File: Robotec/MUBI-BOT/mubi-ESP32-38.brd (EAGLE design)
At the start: 76.5 x 49.5 mm, 20 parts, among them IC1 L293D, IC2 7805T

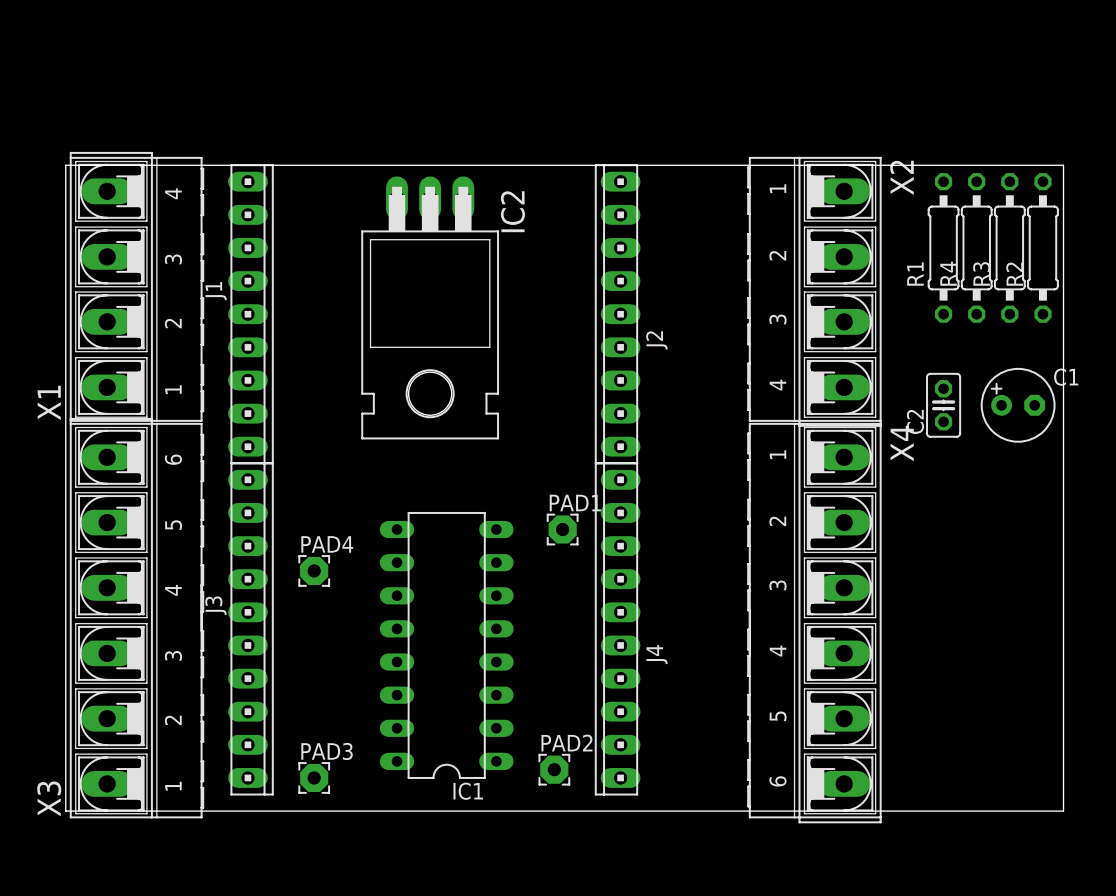
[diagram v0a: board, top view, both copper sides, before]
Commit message: update MUBI-BOT
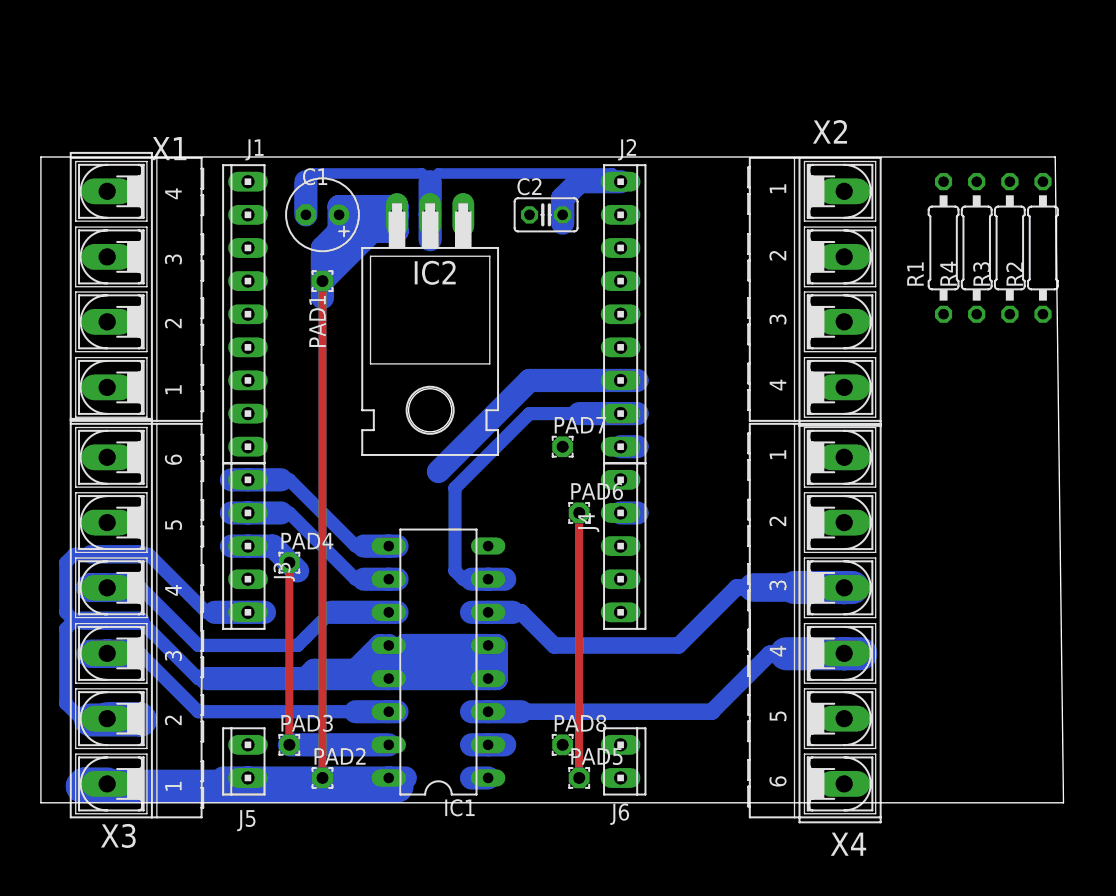
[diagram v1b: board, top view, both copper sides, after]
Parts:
- added J5, J6: (no value), con-amp:10X02MTA
- added PAD5, PAD6, PAD7, PAD8: WIREPAD1,6/0,9, wirepad:1,6/0,9
- J3, J4: device con-amp:10X10MTA -> con-amp:10X05MTA
- PAD1, PAD2, PAD3, PAD4: value WIREPAD2,15/1,0 -> WIREPAD1,6/0,9; device wirepad:2,15/1,0 -> wirepad:1,6/0,9
- moved C1 55.3 mm to (19.7, 45.7), turned to 180 degrees
- moved C2 33.8 mm to (36.8, 45.7), turned to 0 degrees
- moved PAD1 26.5 mm to (19.7, 40.6)
- moved PAD2 17.8 mm to (19.7, 2.54)
- moved J3 6.35 mm to (14.0, 20.3), turned to 90 degrees
- moved J4 6.35 mm to (42.5, 20.3), turned to 270 degrees
- moved PAD3 3.18 mm to (17.1, 5.08)
- moved PAD4 2.01 mm to (17.1, 19.1)
- moved IC1 1.42 mm to (28.6, 11.4)
- moved IC2 1.27 mm to (27.9, 35.6)
- turned J1 to 90 degrees
- turned J2 to 270 degrees
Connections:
- net VCC2 renamed +VBAT
- removed net GND1: IC1.4
- removed net GND2: IC1.5
- removed net GND3: IC1.13
- removed net GND4: IC1.12
- removed net N$1: PAD1.1, PAD2.1
- removed net N$2: PAD3.1, PAD4.1
- removed net VCC1: IC1.16
- new net +3.3V: J1.1
- new net +5V: C1.+, IC1.16, IC2.3, J5.2, PAD1.1, PAD2.1, X3.1
- new net CM11: IC1.2, J2.1, PAD7.1, PAD8.1
- new net CM12: IC1.7, J2.2
- new net CM21: IC1.15, J3.3, PAD3.1, PAD4.1
- new net CM22: IC1.10, J3.2
- new net ENAM1: IC1.1, J4.4, PAD5.1, PAD6.1
- new net ENAM2: IC1.9, J3.1
- new net GND: C1.-, C2.2, IC1.12, IC1.13, IC1.4, IC1.5, IC2.2, J2.3, J2.9, J3.5, X3.2
- new net GPIO23: J2.8
- new net M11: IC1.3, X4.4
- new net M12: IC1.6, X4.3
- new net M21: IC1.14, X3.3
- new net M22: IC1.11, X3.4
- new net N$3: C2.1, IC2.1
- new net SCL: J2.7
- new net SDA: J2.4
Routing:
- net GND: track 0.00 -> 169.0 mm
- net +5V: track 0.00 -> 109.5 mm
- net M12: track 0.00 -> 32.1 mm
- net M11: track 0.00 -> 31.7 mm
- net M22: track 0.00 -> 28.9 mm
- net CM21: track 0.00 -> 27.5 mm
- net CM12: track 0.00 -> 26.8 mm
- net M21: track 0.00 -> 25.4 mm
- net ENAM1: track 0.00 -> 22.9 mm
- net ENAM2: track 0.00 -> 14.8 mm
- net CM22: track 0.00 -> 14.8 mm
- net CM11: track 0.00 -> 3.81 mm
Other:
- board size 76.5 x 49.5 mm -> 78.4 x 49.5 mm

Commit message: update MUBI-BOT
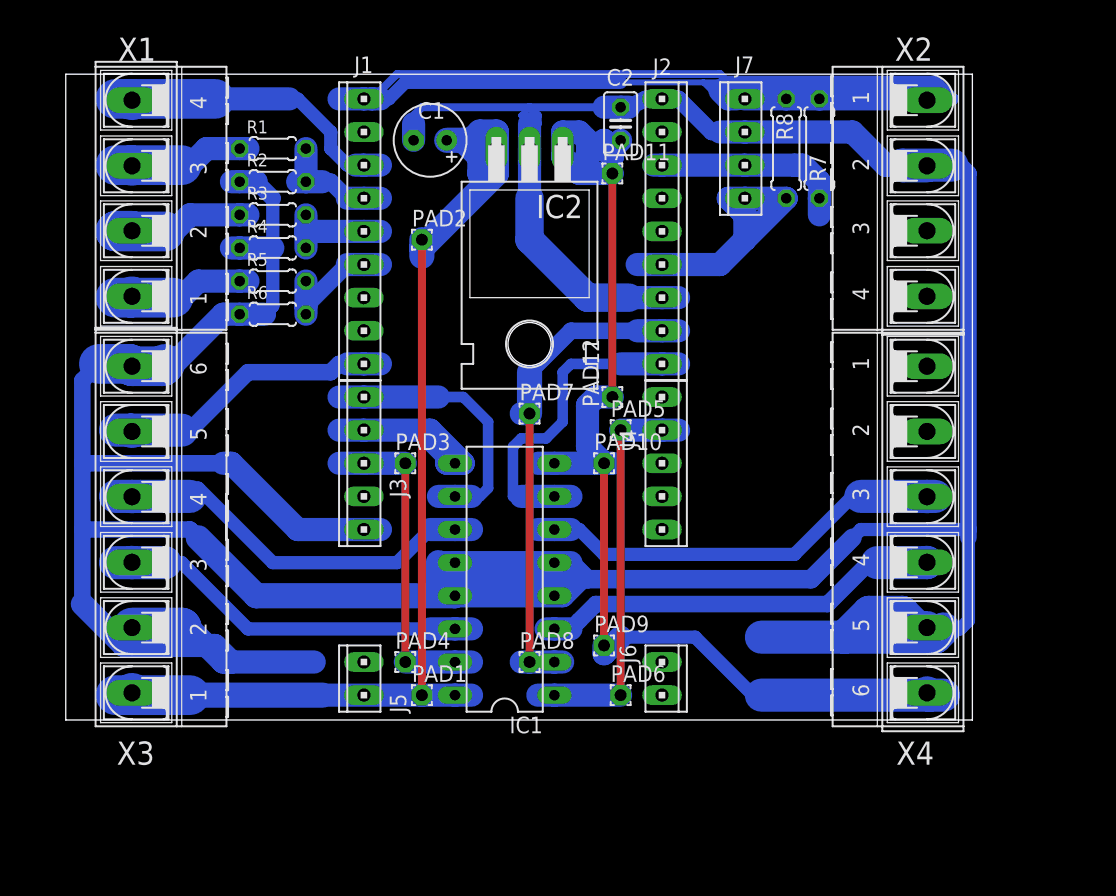
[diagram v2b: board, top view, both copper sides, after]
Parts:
- added J7: (no value), con-amp:10X04MTA
- added PAD10, PAD11, PAD12, PAD9: WIREPAD1,6/0,9, wirepad:1,6/0,9
- added R5, R6: (no value), resistor:0204/5
- added R7, R8: (no value), resistor:0207/7
- R1, R2, R3, R4: device resistor:0207/10 -> resistor:0204/5
- moved R2 59.3 mm to (15.9, 48.3), turned to 0 degrees
- moved R3 56.6 mm to (15.9, 45.7), turned to 0 degrees
- moved R4 54.0 mm to (15.9, 43.2), turned to 0 degrees
- moved R1 52.0 mm to (15.9, 50.8), turned to 0 degrees
- moved PAD2 42.0 mm to (27.3, 43.8)
- moved PAD1 32.7 mm to (27.3, 8.89)
- moved PAD5 26.9 mm to (42.5, 29.2)
- moved PAD3 23.3 mm to (26.0, 26.7)
- moved PAD6 14.3 mm to (42.5, 8.89)
- moved PAD4 11.7 mm to (26.0, 11.4)
- moved J1 10.9 mm to (22.9, 44.5)
- moved J3 10.9 mm to (22.9, 26.7)
- moved J5 10.9 mm to (22.9, 10.2)
- moved C1 10.0 mm to (27.9, 51.4)
- moved X2 9.44 mm to (66.0, 47.0)
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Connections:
- removed net GPIO23: J2.8
- new net AUX2: J1.9, X3.5
- new net N$1: R1.1, X1.3
- new net N$2: R3.1, X1.2
- new net N$4: J1.3, X1.4
- new net USON1: J1.4, R1.2, R2.2
- new net USON2: J1.5, R3.2, R4.2
- new net USON3: J1.6, R5.2, R6.2
- net +3.3V: now also J7.1, R7.2, R8.2, X2.1
- net +VBAT: now also C2.1, IC2.1, PAD10.1, PAD11.1, PAD12.1, PAD9.1, X4.6
- net CM11: now also J2.2; no longer J2.1
- net CM12: now also J2.1; no longer J2.2
- net CM22: now also J3.1; no longer J3.2
- net ENAM2: now also J3.2; no longer J3.1
- net GND: now also J7.2, R2.1, R4.1, R6.1, X2.2, X3.6, X4.5
- net N$3: now also R5.1, X1.1; no longer C2.1, IC2.1
- net SCL: now also J7.3, R7.1, X2.3
- net SDA: now also J7.4, R8.1, X2.4
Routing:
- net GND: track 169.0 -> 340.3 mm
- net +3.3V: track 0.00 -> 110.5 mm
- net +VBAT: track 0.00 -> 88.7 mm
- net CM11: track 3.81 -> 38.8 mm
- net +5V: track 109.5 -> 84.6 mm
- net N$4: track 0.00 -> 23.3 mm
- net SDA: track 0.00 -> 23.0 mm
- net AUX2: track 0.00 -> 22.6 mm
- net SCL: track 0.00 -> 15.8 mm
- net N$2: track 0.00 -> 12.0 mm
- net N$3: track 0.00 -> 10.8 mm
- net N$1: track 0.00 -> 10.8 mm
- net USON3: track 0.00 -> 9.57 mm
- net USON1: track 0.00 -> 9.42 mm
- net ENAM1: track 22.9 -> 31.1 mm
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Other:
- board size 78.4 x 49.5 mm -> 69.5 x 49.5 mm
